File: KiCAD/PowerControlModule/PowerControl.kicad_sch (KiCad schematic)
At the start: 58 parts, among them J1 DF1B-2S-2.5R, J2 DF1B-2S-2.5R, Q1 AO3401A, Q10 AO3401A, Q11 Si4162DY, Q12 Si4162DY, Q2 AO3401A, Q3 AO3400A, Q4 AO3401A, Q5 AO3401A, Q6 AO3401A, Q7 AO3401A, Q9 AO3401A, U11 LTC3119, U3 INA228, U4 INA228, U5 LTC4353, U6 INA228

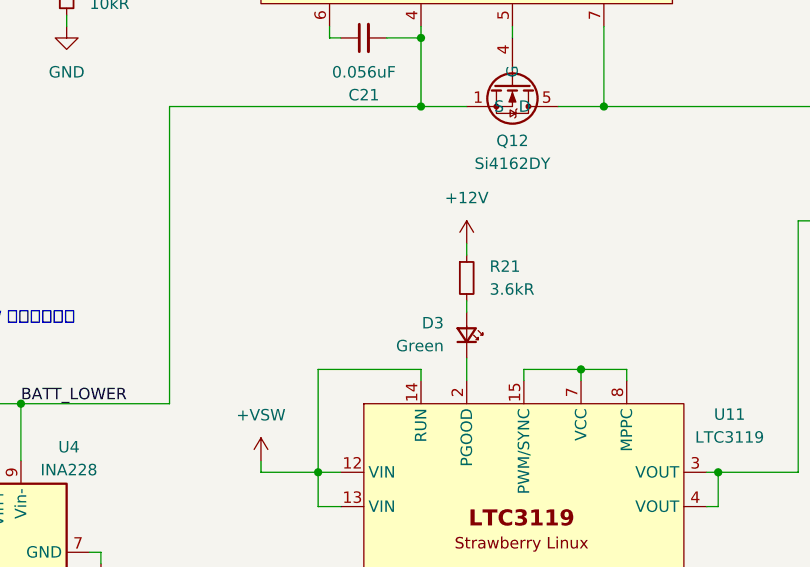
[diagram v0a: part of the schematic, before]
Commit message: 修正した．発注する．
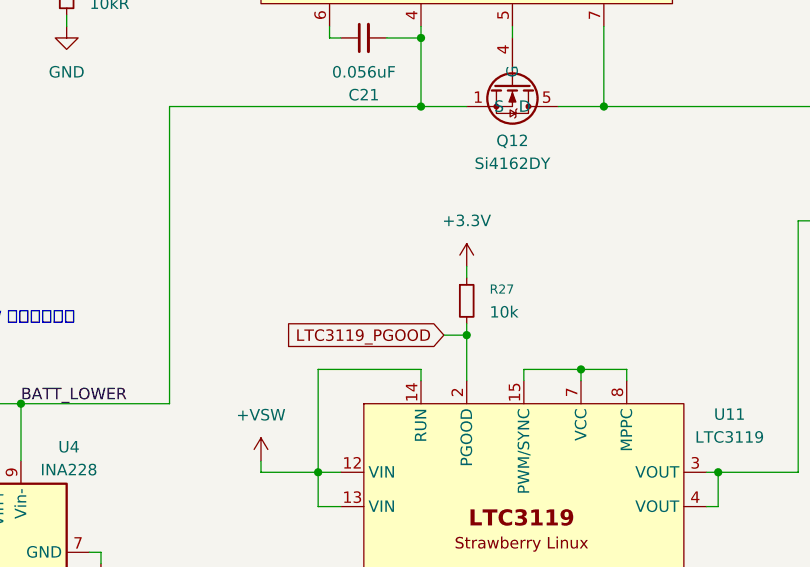
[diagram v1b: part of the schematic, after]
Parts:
- removed D3: Green, LED_SMD:LED_0603_1608Metric_Pad1.05x0.95mm_HandSolder, symbol Device:LED_Small
- removed R21: 3.6kR, Resistor_SMD:R_0603_1608Metric_Pad0.98x0.95mm_HandSolder, symbol Device:R_Small
- added R27: 10k, Resistor_SMD:R_0603_1608Metric, symbol Device:R_Small
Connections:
- net +3.3V: now also R27.1
- net LTC3119_PGOOD: now reaches U11.2 (PGOOD)
- net LTC3119_PGOOD: now also R27.2
